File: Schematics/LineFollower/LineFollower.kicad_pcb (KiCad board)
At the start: 2 copper layers, 1 part, among them U1 STM32F405VGTx

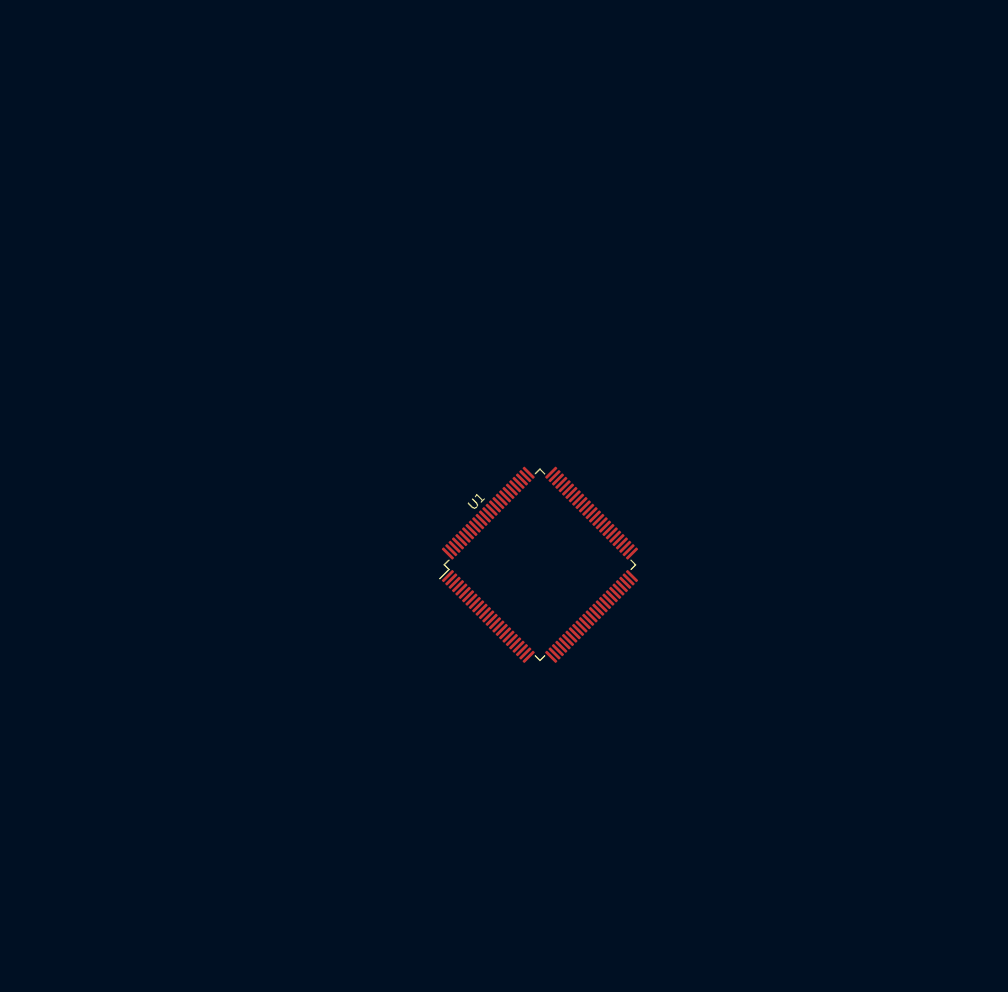
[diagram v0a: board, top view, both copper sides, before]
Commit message: Uploaded V1.0 of PCB
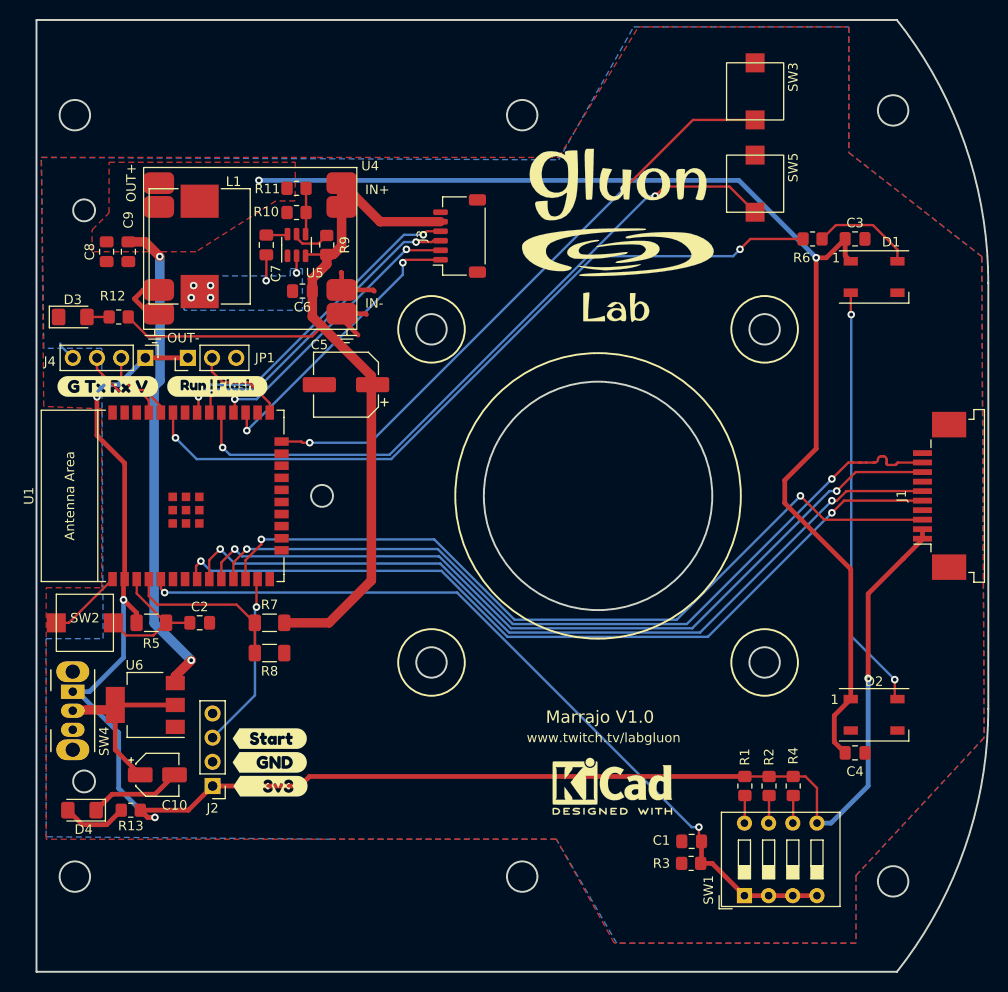
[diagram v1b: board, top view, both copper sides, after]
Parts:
- added C1: 100nF, Capacitor_SMD:C_0805_2012Metric_Pad1.18x1.45mm_HandSolder, F.Cu at (163.9, 128.7)
- added C10: C_Polarized_US, Capacitor_SMD:CP_Elec_4x5.3, F.Cu at (107.7, 121.7)
- added C2: 100nF, Capacitor_SMD:C_0805_2012Metric_Pad1.18x1.45mm_HandSolder, F.Cu at (112.2, 105.7)
- added C3: 100nF, Capacitor_SMD:C_0805_2012Metric_Pad1.18x1.45mm_HandSolder, F.Cu at (181.0, 65.4)
- added C4: 100nF, Capacitor_SMD:C_0805_2012Metric_Pad1.18x1.45mm_HandSolder, F.Cu at (181.0, 119.4)
- added C5: 100u, Capacitor_SMD:CP_Elec_6.3x5.4, F.Cu at (127.5, 80.7)
- added C6: 22u, Capacitor_SMD:C_0805_2012Metric_Pad1.18x1.45mm_HandSolder, F.Cu at (123.0, 70.9)
- added C7: 100n, Capacitor_SMD:C_0805_2012Metric_Pad1.18x1.45mm_HandSolder, F.Cu at (119.2, 66.0)
- added C8: 22u, Capacitor_SMD:C_0805_2012Metric_Pad1.18x1.45mm_HandSolder, F.Cu at (102.4, 66.7)
- added C9: 22u, Capacitor_SMD:C_0805_2012Metric_Pad1.18x1.45mm_HandSolder, F.Cu at (104.7, 66.7)
- added D1: WS2812B, LED_SMD:LED_WS2812B_PLCC4_5.0x5.0mm_P3.2mm, F.Cu at (183.0, 69.4)
- added D2: WS2812B, LED_SMD:LED_WS2812B_PLCC4_5.0x5.0mm_P3.2mm, F.Cu at (183.0, 115.4)
- added D3: vBatt, LED_SMD:LED_1206_3216Metric_Pad1.42x1.75mm_HandSolder, F.Cu at (98.8, 73.6)
- added D4: 3v3, LED_SMD:LED_1206_3216Metric_Pad1.42x1.75mm_HandSolder, F.Cu at (99.8, 125.4)
- added G***: LOGO, GluonLib:LogoGluon_25mm, F.Cu at (156.0, 64.4)
- added J1: Morro, Connector_FFC-FPC:TE_1-84952-0_1x10-1MP_P1.0mm_Horizontal, F.Cu at (189.9, 92.4)
- added J2: StartModule, Connector_PinHeader_2.54mm:PinHeader_1x04_P2.54mm_Vertical, F.Cu at (113.5, 122.9)
- added J3: 4en1, Connector_JST:JST_SH_SM06B-SRSS-TB_1x06-1MP_P1.00mm_Horizontal, F.Cu at (139.5, 65.1)
- added J4: UART, Connector_PinHeader_2.54mm:PinHeader_1x04_P2.54mm_Vertical, F.Cu at (106.5, 77.9)
- added JP1: BOOT_SELECT, Connector_PinHeader_2.54mm:PinHeader_1x03_P2.54mm_Vertical, F.Cu at (110.9, 77.9)
- added L1: 3u3, Inductor_SMD:L_Chilisin_BMRF00101040, F.Cu at (112.2, 66.2)
- added R1: 4k7, Resistor_SMD:R_0805_2012Metric_Pad1.20x1.40mm_HandSolder, F.Cu at (169.5, 122.9)
- added R10: 10k, Resistor_SMD:R_0805_2012Metric_Pad1.20x1.40mm_HandSolder, F.Cu at (122.4, 62.6)
- added R11: 54k9, Resistor_SMD:R_0805_2012Metric_Pad1.20x1.40mm_HandSolder, F.Cu at (122.4, 60.1)
- added R12: 4k7, Resistor_SMD:R_0805_2012Metric_Pad1.20x1.40mm_HandSolder, F.Cu at (103.7, 73.6)
- added R13: 1k, Resistor_SMD:R_0805_2012Metric_Pad1.20x1.40mm_HandSolder, F.Cu at (104.9, 125.4)
- added R2: 2k2, Resistor_SMD:R_0805_2012Metric_Pad1.20x1.40mm_HandSolder, F.Cu at (172.0, 122.9)
- added R3: 2k2, Resistor_SMD:R_0805_2012Metric_Pad1.20x1.40mm_HandSolder, F.Cu at (163.8, 131.0)
- added R4: 1k, Resistor_SMD:R_0805_2012Metric_Pad1.20x1.40mm_HandSolder, F.Cu at (174.5, 122.9)
- added R5: 10k, Resistor_SMD:R_1206_3216Metric_Pad1.30x1.75mm_HandSolder, F.Cu at (107.1, 105.7)
- added R6: 470, Resistor_SMD:R_0805_2012Metric_Pad1.20x1.40mm_HandSolder, F.Cu at (176.6, 65.4)
- added R7: 47k, Resistor_SMD:R_1206_3216Metric_Pad1.30x1.75mm_HandSolder, F.Cu at (119.5, 105.7)
- added R8: 10k, Resistor_SMD:R_1206_3216Metric_Pad1.30x1.75mm_HandSolder, F.Cu at (119.5, 108.9)
- added R9: 10k, Resistor_SMD:R_0805_2012Metric_Pad1.20x1.40mm_HandSolder, F.Cu at (125.5, 66.0)
- added REF**: KiCad-Logo2_5mm_SilkScreen, Symbol:KiCad-Logo2_5mm_SilkScreen, F.Cu at (155.5, 122.9)
- added SW1: SW_DIP_x04, Button_Switch_THT:SW_DIP_SPSTx04_Slide_9.78x12.34mm_W7.62mm_P2.54mm, F.Cu at (169.4, 134.4)
- added SW2: SW_Push, switches:SKPMANE010 _Silicone_6x6mm, F.Cu at (100.1, 105.7)
- added SW3: Push2, switches:SKPMANE010 _Silicone_6x6mm, F.Cu at (170.5, 49.9)
- added SW4: SW_Push_SPDT, switches:SS12D07VG2, F.Cu at (98.8, 113.0)
- added SW5: Start, switches:SKPMANE010 _Silicone_6x6mm, F.Cu at (170.5, 59.6)
- added U4: ~, modulos:5v-Reg, F.Cu at (117.5, 66.4)
- added U5: TPS563201, Package_TO_SOT_SMD:SOT-23-6, F.Cu at (122.4, 66.0)
- added U6: AMS1117-3.3, Package_TO_SOT_SMD:SOT-223-3_TabPin2, F.Cu at (106.5, 114.4)
- added kibuzzard-65DCBE20: G***, kibuzzard-65DCBE20, F.Cu at (119.5, 117.9)
- added kibuzzard-65DCBE24: G***, kibuzzard-65DCBE24, F.Cu at (119.5, 120.4)
- added kibuzzard-65DCBE28: G***, kibuzzard-65DCBE28, F.Cu at (119.6, 122.9)
- added kibuzzard-65DCBF71: G***, kibuzzard-65DCBF71, F.Cu at (114.0, 80.9)
- added kibuzzard-65DCBFCA: G***, kibuzzard-65DCBFCA, F.Cu at (102.5, 80.9)
- U1: value STM32F405VGTx -> ESP32-WROOM-E; footprint Package_QFP:LQFP-100_14x14mm_P0.5mm -> Espressif:ESP32-WROOM-32E
- moved U1 38.6 mm to (110.0, 92.4), turned to 90 degrees
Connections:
- U1 pad 1: unconnected-(U1-PE2-Pad1) -> GND
- U1 pad 10: Net-(U1-VSS-Pad10) -> /SCL
- U1 pad 11: unconnected-(U1-VDD-Pad11) -> /SDA
- U1 pad 12: unconnected-(U1-PH0-Pad12) -> /MOSFET_PWM
- U1 pad 13: unconnected-(U1-PH1-Pad13) -> /START
- U1 pad 15: unconnected-(U1-PC0-Pad15) -> GND
- U1 pad 2: unconnected-(U1-PE3-Pad2) -> +3V3
- U1 pad 24: unconnected-(U1-PA1-Pad24) -> Net-(U1-ADC2_CH2/GPIO2)
- U1 pad 25: unconnected-(U1-PA2-Pad25) -> /BOOT_SELECT
- U1 pad 27: Net-(U1-VSS-Pad10) -> /MOTOR_1
- U1 pad 28: unconnected-(U1-VDD-Pad28) -> /MOTOR_2
- U1 pad 29: unconnected-(U1-PA4-Pad29) -> Net-(U1-GPIO5)
- U1 pad 3: unconnected-(U1-PE4-Pad3) -> Net-(U1-EN/CHIP_PU)
- U1 pad 30: unconnected-(U1-PA5-Pad30) -> /MOTOR_3
- U1 pad 31: unconnected-(U1-PA6-Pad31) -> /MOTOR_4
- U1 pad 33: unconnected-(U1-PC4-Pad33) -> /RGB_PIN
- U1 pad 34: unconnected-(U1-PC5-Pad34) -> /UART_RX
- U1 pad 35: unconnected-(U1-PB0-Pad35) -> /UART_TX
- U1 pad 36: unconnected-(U1-PB1-Pad36) -> /ENC_1A
- U1 pad 37: unconnected-(U1-PB2-Pad37) -> /ENC_1B
- U1 pad 38: unconnected-(U1-PE7-Pad38) -> GND
- U1 pad 39: unconnected-(U1-PE8-Pad39) -> GND
- U1 pad 4: unconnected-(U1-PE5-Pad4) -> /V_BATT_SENSE
- U1 pad 5: unconnected-(U1-PE6-Pad5) -> /CONFIG
- U1 pad 6: unconnected-(U1-VBAT-Pad6) -> /ENC_2A
- U1 pad 7: unconnected-(U1-PC13-Pad7) -> /ENC_2B
- U1 pad 8: unconnected-(U1-PC14-Pad8) -> /V1
- U1 pad 9: unconnected-(U1-PC15-Pad9) -> /V2
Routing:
- net +3V3: track 0.00 -> 182.5 mm, vias 0 -> 4
- net +5V: track 0.00 -> 177.2 mm, vias 0 -> 4
- net /V_BATT: track 0.00 -> 95.0 mm
- net /V2: track 0.00 -> 87.2 mm, vias 0 -> 2
- net /V1: track 0.00 -> 87.2 mm, vias 0 -> 2
- net /SCL: track 0.00 -> 86.2 mm, vias 0 -> 2
- net /SDA: track 0.00 -> 86.2 mm, vias 0 -> 2
- net /CONFIG: track 0.00 -> 85.5 mm, vias 0 -> 2
- net /MOSFET_PWM: track 0.00 -> 84.3 mm, vias 0 -> 2
- net /RGB_PIN: track 0.00 -> 79.2 mm, vias 0 -> 2
- net Net-(U1-GPIO5): track 0.00 -> 72.8 mm, vias 0 -> 2
- net Net-(U1-ADC2_CH2/GPIO2): track 0.00 -> 63.8 mm, vias 0 -> 2
- net Net-(D1-DOUT): track 0.00 -> 44.7 mm, vias 0 -> 2
- net GND: track 0.00 -> 36.8 mm
- net /MOTOR_4: track 0.00 -> 34.4 mm, vias 0 -> 2
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- added copper zone on F.Cu, net +5V
- added copper zone on B.Cu, net GND
- added copper zone on F.Cu, net GND
- added copper zone on B.Cu, net Net-(U5-SW)
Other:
- board outline added: 100 x 100 mm
- board text added: "Gracias a: spuertes araba_st andygm_ zurano_ carlosbetdev 56knews gorn6_ david_wiki humiltat pipermind txusev supersonic2510 raupulus sergivv gordon_clark enlopa devjoseantonio bern245 alnaumiwebs blacai mikalet_ rafaromevi dhontecillas adiiran dcorraliza dielek arminio_ movich4 diegomallo sistemasitpro kerneltron patoovf dragore76 teoreding bark12 andrewsc08 siodh 20_leunam elchulodelanieve hack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"
- board text added: "Marrajo V1.0"
- board text added: "www.twitch.tv/labgluon"
